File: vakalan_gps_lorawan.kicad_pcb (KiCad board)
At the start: 2 copper layers, 147.5 x 90.1 mm, 64 parts, among them J1 Conn_01x08_Male, U1 BMM150, U2 TPS62A01DRLR_, U3 18650, U4 18650, U5 18650, U6 18650, U7 18650, U8 18650

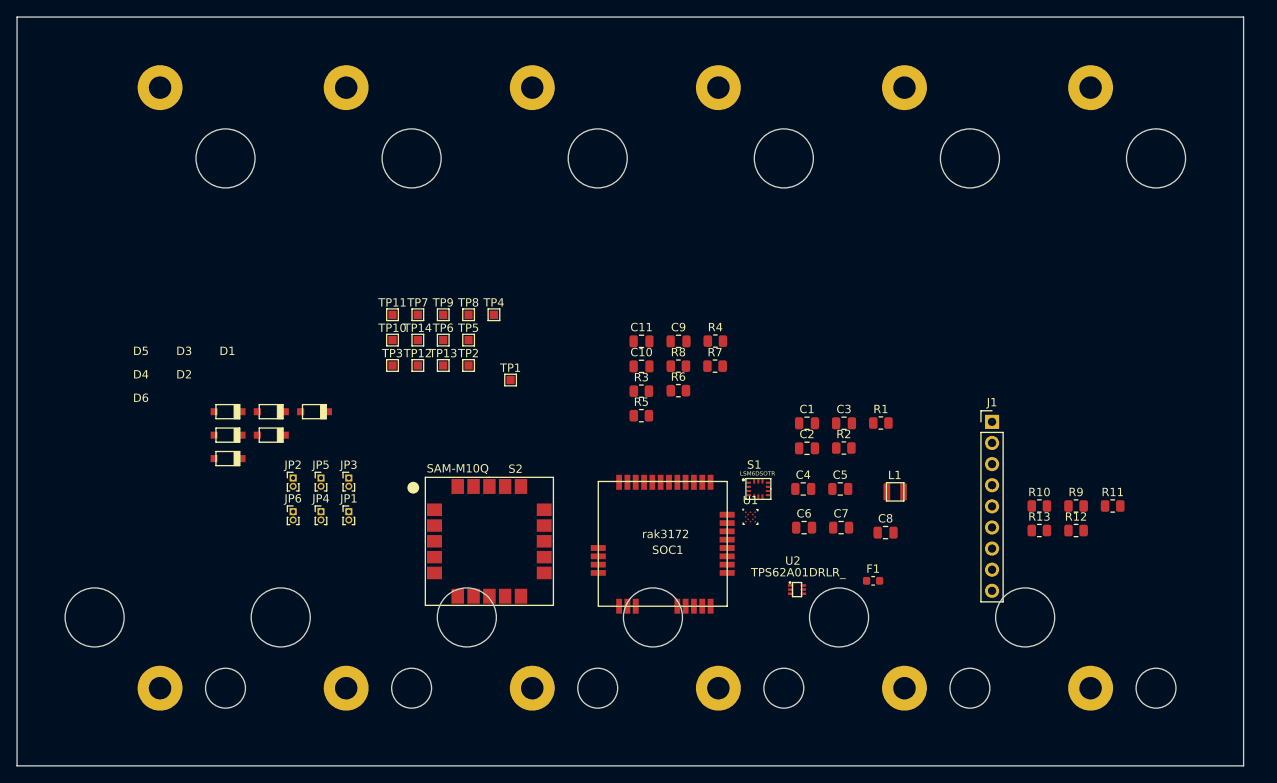
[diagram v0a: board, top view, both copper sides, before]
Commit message: .
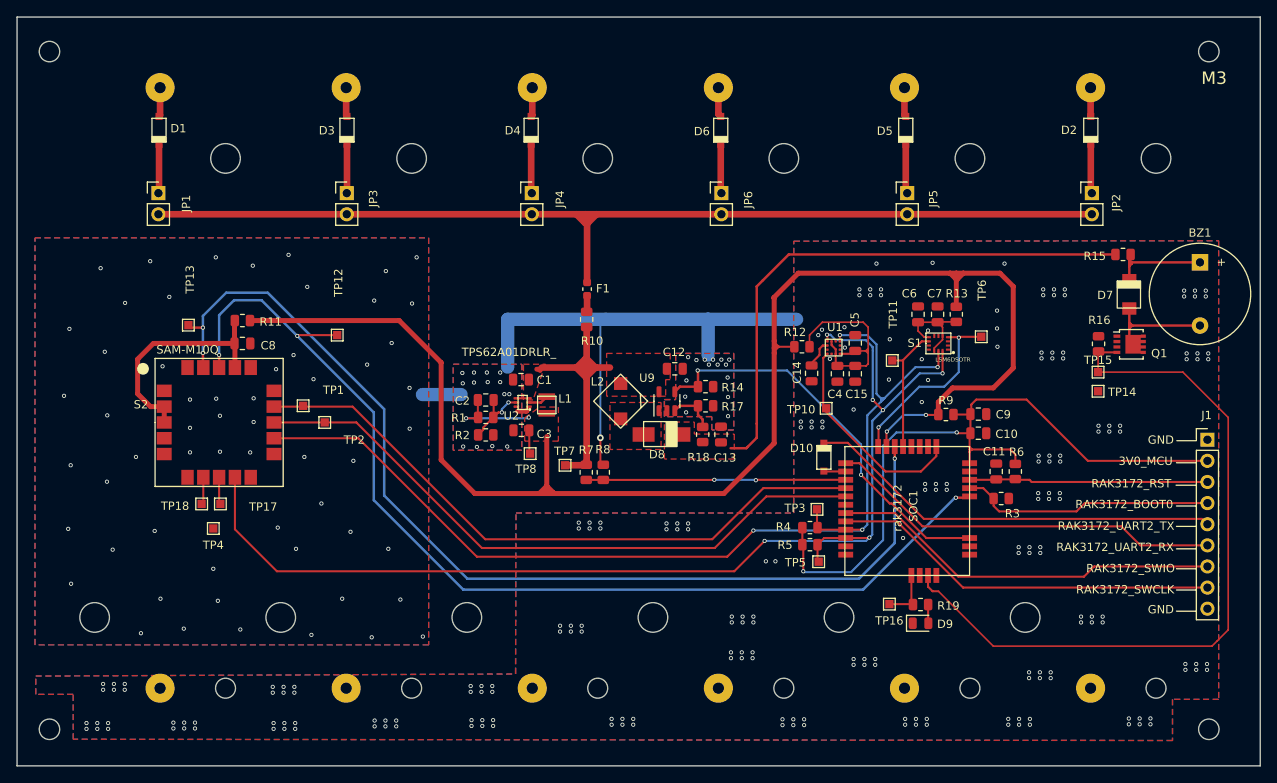
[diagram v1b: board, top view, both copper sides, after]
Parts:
- removed TP9: TestPoint_Probe, TestPoint:TestPoint_Pad_1.0x1.0mm
- added BZ1: Buzzer, Buzzer_Beeper:Buzzer_12x9.5RM7.6, F.Cu at (190.3, 85.8)
- added C12: 4.7uF, Capacitor_SMD:C_0805_2012Metric, F.Cu at (127.1, 98.7)
- added C13: 1uF, Capacitor_SMD:C_0805_2012Metric, F.Cu at (132.7, 106.5)
- added C14: 220Nf, Capacitor_SMD:C_0805_2012Metric, F.Cu at (143.6, 99.2)
- added C15: 0.1uF, Capacitor_SMD:C_0805_2012Metric, F.Cu at (148.8, 99.2)
- added D10: BAT54G, vakalan:BAT54G, F.Cu at (145.1, 109.2)
- added D7: D, vakalan:FM4006, F.Cu at (181.8, 89.6)
- added D8: D, vakalan:SS14, F.Cu at (124.3, 106.5)
- added D9: LED, LED_SMD:LED_0805_2012Metric, F.Cu at (156.7, 129.2)
- added L2: 10uH, vakalan:CDRH4D16-100M, F.Cu at (120.5, 102.7)
- added Q1: BUK9M11-40EX, Package_TO_SOT_SMD:LFPAK33, F.Cu at (181.8, 95.7)
- added R14: 10k, Resistor_SMD:R_0805_2012Metric, F.Cu at (130.8, 100.8)
- added R15: 0, Resistor_SMD:R_0805_2012Metric, F.Cu at (181.0, 84.9)
- added R16: 10k, Resistor_SMD:R_0805_2012Metric, F.Cu at (178.1, 95.7)
- added R17: 120k, Resistor_SMD:R_0805_2012Metric, F.Cu at (130.8, 103.1)
- added R18: 1M, Resistor_SMD:R_0805_2012Metric, F.Cu at (130.4, 106.5)
- added R19: 4.7k, Resistor_SMD:R_0805_2012Metric, F.Cu at (156.7, 127.0)
- added TP15: TestPoint_Probe, TestPoint:TestPoint_Pad_1.0x1.0mm, F.Cu at (178.0, 99.0)
- added TP16: TestPoint_Probe, TestPoint:TestPoint_Pad_1.0x1.0mm, F.Cu at (152.9, 127.0)
- added TP17: TestPoint_Probe, TestPoint:TestPoint_Pad_1.0x1.0mm, F.Cu at (72.5, 114.9)
- added TP18: TestPoint_Probe, TestPoint:TestPoint_Pad_1.0x1.0mm, F.Cu at (70.2, 114.9)
- added U9: AP3012, Package_TO_SOT_SMD:SOT-23-5, F.Cu at (126.2, 102.5)
- C4: value 0.1uF -> 10uF
- JP1, JP2, JP3, JP4, JP5, JP6: footprint Connector_PinHeader_1.00mm:PinHeader_1x02_P1.00mm_Vertical -> Connector_PinHeader_2.54mm:PinHeader_1x02_P2.54mm_Vertical
- U1: value BMM150 -> IIS2MDCTR; footprint Package_CSP:WLCSP-12_1.56x1.56mm_P0.4mm -> vakalan:IIS2MDCTR
- moved R11 107.0 mm to (75.1, 92.8), turned to 180 degrees
- moved D2 105.1 mm to (177.1, 70.0), turned to -90 degrees
- moved JP2 102.0 mm to (177.2, 77.5)
- moved D5 88.2 mm to (154.8, 70.0), turned to -90 degrees
- moved TP14 82.0 mm to (178.0, 101.3)
- moved C8 80.6 mm to (75.1, 95.6)
- moved JP5 78.4 mm to (155.1, 77.5)
- moved D6 71.2 mm to (132.6, 70.0), turned to -90 degrees
- moved TP6 64.7 mm to (163.9, 94.8)
- moved JP6 64.2 mm to (132.7, 77.5)
- moved TP11 60.4 mm to (153.2, 97.7)
- moved R10 58.9 mm to (116.5, 92.7), turned to -90 degrees
- moved TP3 53.9 mm to (144.2, 115.5)
- moved TP10 52.8 mm to (145.3, 103.4)
- moved D4 51.7 mm to (109.8, 70.0), turned to -90 degrees
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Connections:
- J1 pad 3: RAK3172_UART2_TX -> RAK3172_RST
- J1 pad 4: RAK3172_UART2_RX -> RAK3172_BOOT0
- J1 pad 5: RAK3172_SWIO -> RAK3172_UART2_TX
- J1 pad 6: RAK3172_SWCLK -> RAK3172_UART2_RX
- J1 pad 7: RAK3172_BOOT0 -> RAK3172_SWIO
- J1 pad 8: RAK3172_RST -> RAK3172_SWCLK
- S2 pad 7: unconnected-(S2-Pad7) -> Net-(S2-Pad7)
- S2 pad 8: unconnected-(S2-Pad8) -> Net-(S2-Pad8)
- SOC1 pad 13: unconnected-(SOC1-Pad13) -> LED
- SOC1 pad 15: unconnected-(SOC1-Pad15) -> BUZZER
- SOC1 pad 19: unconnected-(SOC1-Pad19) -> AP3015_SHDN
- SOC1 pad 2: RAK3172_UART2_TX -> Net-(D10-Pad1)
- SOC1 pad 20: M10Q_EXINT -> M10Q_RESET_N
- SOC1 pad 25: BMM150_INT -> IIS2MDCTR_INT
- SOC1 pad 26: BMM150_DRDY -> unconnected-(SOC1-Pad26)
- SOC1 pad 30: M10Q_RESET_N -> M10Q_EXINT
- TP10 pad 1: BMM150_INT -> IIS2MDCTR_INT
- TP12 pad 1: M10Q_EXINT -> M10Q_RESET_N
- TP13 pad 1: M10Q_RESET_N -> M10Q_EXINT
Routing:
- net ADC_REF: track 0.00 -> 194.1 mm, vias 0 -> 4
- net SDA: track 0.00 -> 137.7 mm, vias 0 -> 6
- net M10Q_RESET_N: track 0.00 -> 127.4 mm, vias 0 -> 3
- net M10Q_EXINT: track 0.00 -> 126.2 mm, vias 0 -> 3
- net SCL: track 0.00 -> 126.0 mm, vias 0 -> 4
- net Net-(F1-Pad1): track 0.00 -> 123.9 mm
- net BUZZER: track 0.00 -> 89.6 mm
- net +3V0_MCU: track 0.00 -> 87.7 mm, vias 0 -> 2
- net M10Q_UART_RX: track 0.00 -> 78.0 mm
- net M10Q_UART_TX: track 0.00 -> 77.6 mm
- net GND: track 0.00 -> 69.1 mm, vias 0 -> 307
- net +12V: track 0.00 -> 66.6 mm
- net RAK3172_UART2_TX: track 0.00 -> 50.4 mm
- net AP3015_SHDN: track 0.00 -> 48.2 mm, vias 0 -> 2
- net RAK3172_UART2_RX: track 0.00 -> 47.6 mm
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- added copper zone on F.Cu, net +12V
- added copper zone on F.Cu, net ADC_REF
- added copper zone on B.Cu, net GND
- added copper zone on F.Cu, net GND
- added copper zone on F.Cu, net Net-(C1-Pad1)
- added copper zone on F.Cu, net Net-(D8-Pad1)
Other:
- board size 147.5 x 90.1 mm -> 149.5 x 90.1 mm
- board text added: "3V0_MCU"
- board text added: "GND"
- board text added: "M3"
- board text added: "RAK3172_BOOT0"
- board text added: "RAK3172_RST"
- board text added: "RAK3172_SWCLK"
- board text added: "RAK3172_SWIO"
- board text added: "RAK3172_UART2_RX"
- board text added: "RAK3172_UART2_TX"
